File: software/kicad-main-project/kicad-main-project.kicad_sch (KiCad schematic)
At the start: 24 parts, among them J1 MOTOR_A, J2 MOTOR_B, SW1 SW_Push, SW2 SW_Push, SW3 SW_Push, SW4 SW_Push, U1 ESP32-DevKitC, U2 AMS117-5V, U3 TB6612FNG, U4 GP2Y0A02YK0F_1, U5 GP2Y0A02YK0F_2, U6 LCD-I2C, U7 CH340E

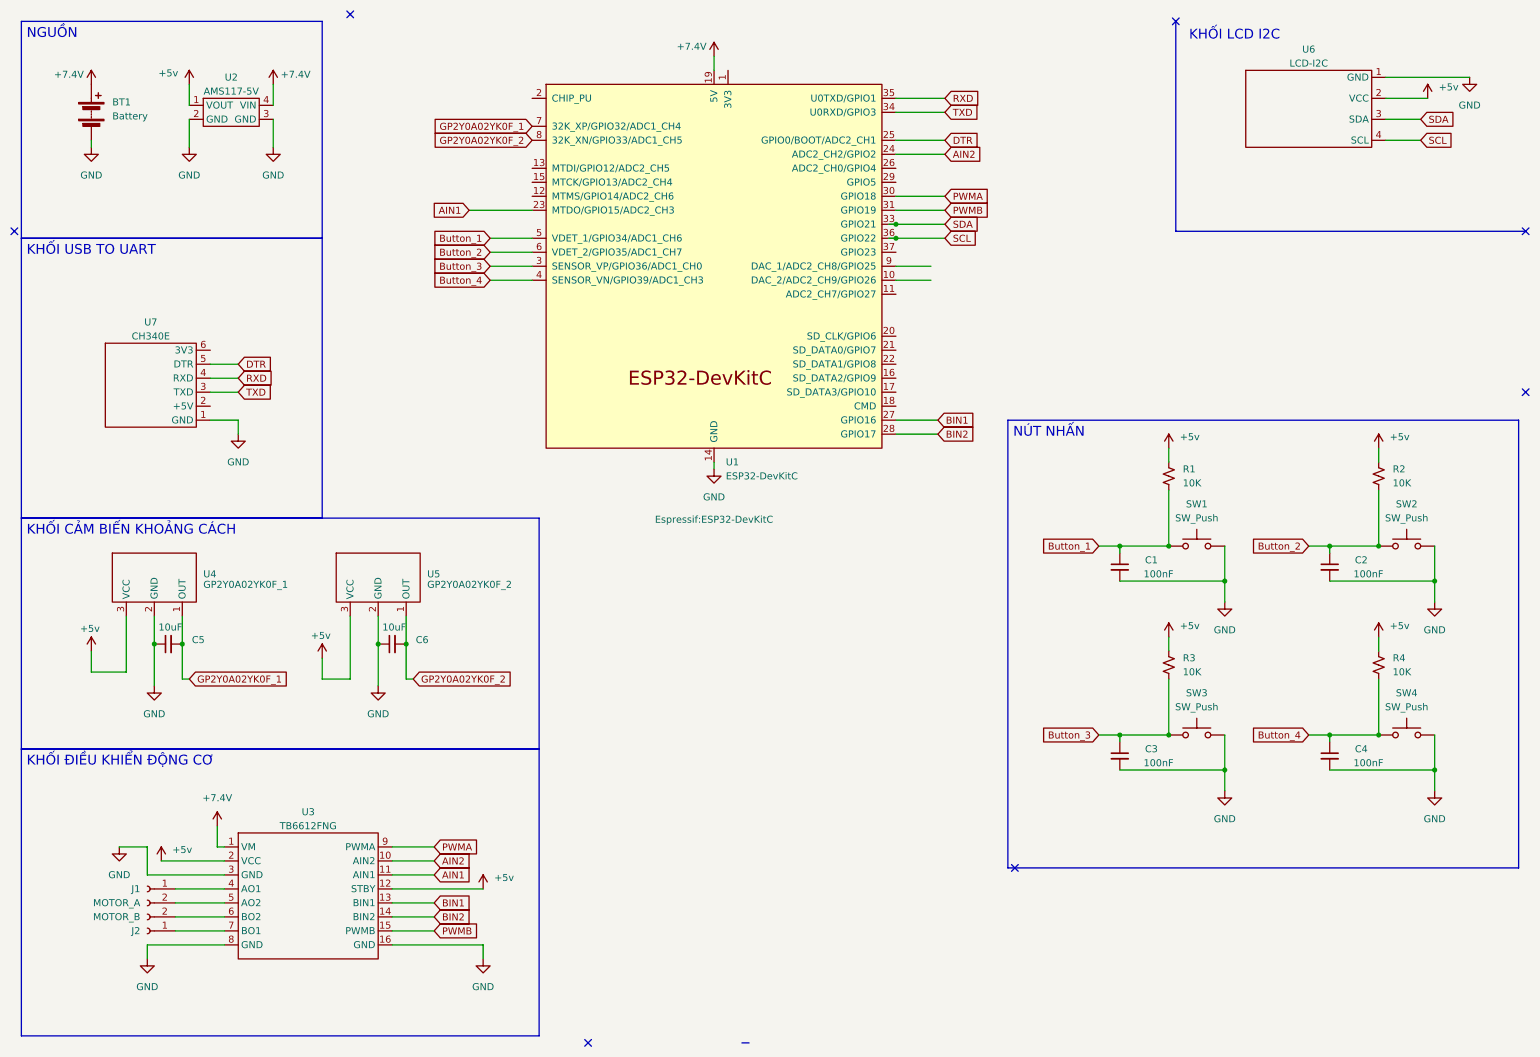
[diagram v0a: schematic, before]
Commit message: update gerber + bom + image_
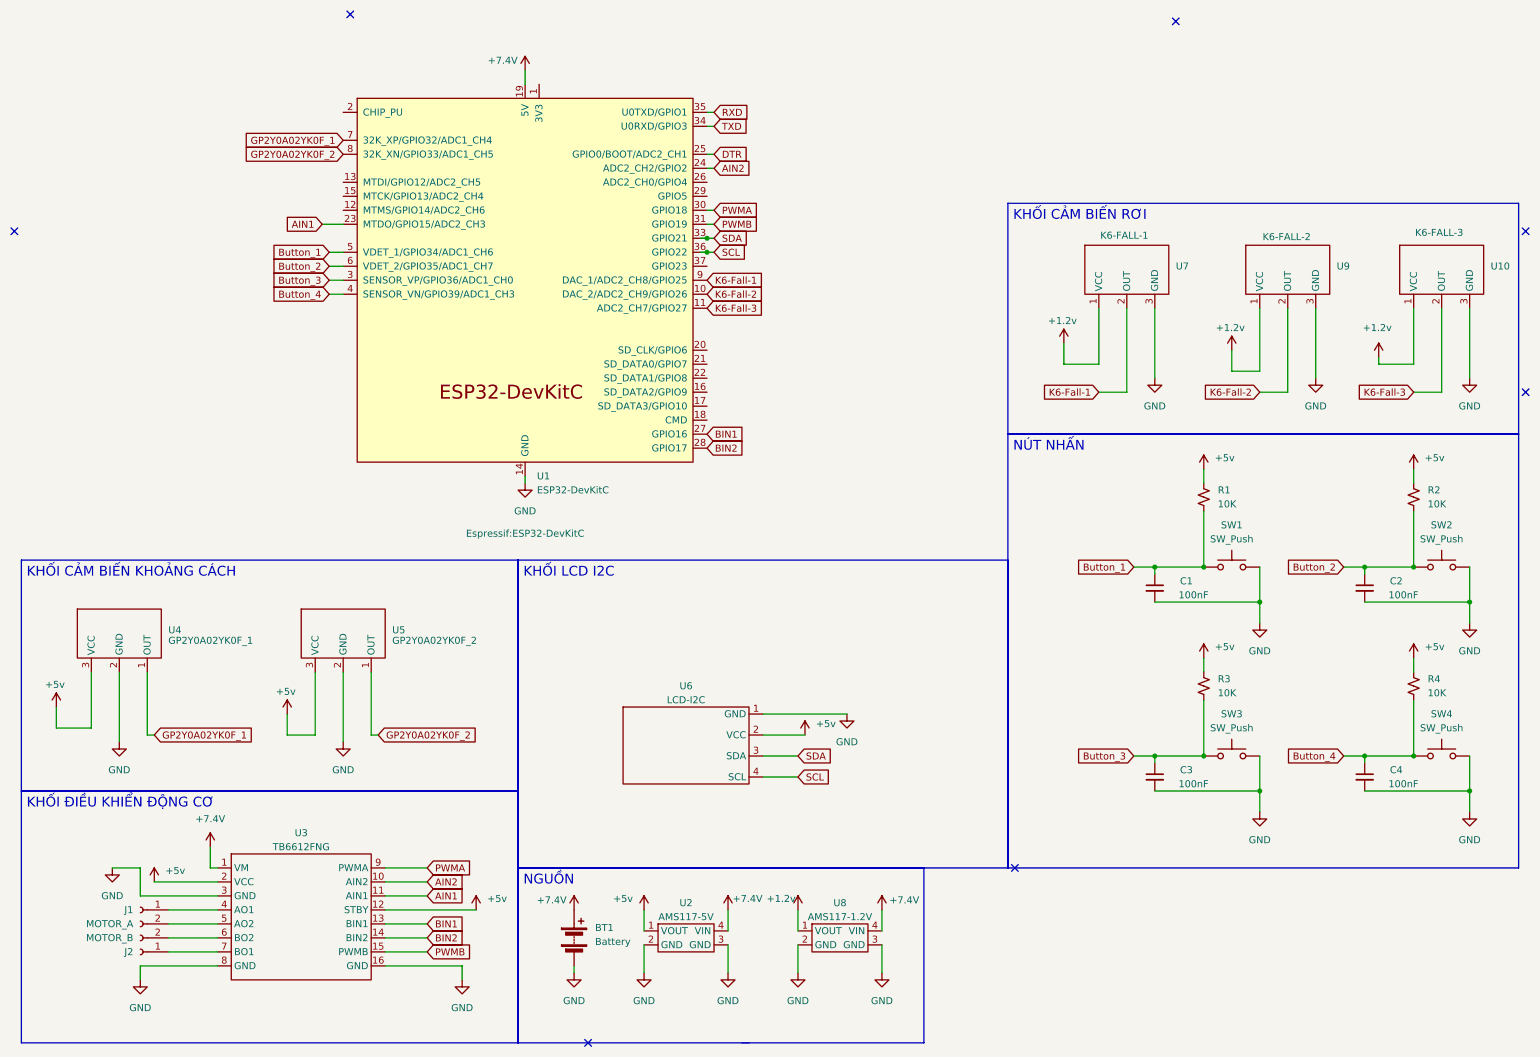
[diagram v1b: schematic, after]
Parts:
- removed C5, C6: 10uF, Capacitor_THT:C_Disc_D3.0mm_W1.6mm_P2.50mm, symbol Device:C_Small
- removed U7: CH340E, myCH340e:Untitled, symbol myCH340E:CH340E
- added U10: K6-FALL-3, Connector_JST:JST_XH_S3B-XH-A-1_1x03_P2.50mm_Horizontal, symbol myK6-Fall:K6-Fall
- added U7: K6-FALL-1, Connector_JST:JST_XH_S3B-XH-A-1_1x03_P2.50mm_Horizontal, symbol myK6-Fall:K6-Fall
- added U8: AMS117-1.2V, myAMS117-5V:Untitled, symbol myAMS117-1V2-Module:myAMS117-1V2
- added U9: K6-FALL-2, Connector_JST:JST_XH_S3B-XH-A-1_1x03_P2.50mm_Horizontal, symbol myK6-Fall:K6-Fall
- R1, R2, R3, R4: footprint Resistor_THT:R_Axial_DIN0617_L17.0mm_D6.0mm_P25.40mm_Horizontal -> Resistor_THT:R_Axial_DIN0204_L3.6mm_D1.6mm_P2.54mm_Vertical
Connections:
- net +7.4V: now also U8.4 (VIN)
- net GND: now also U10.3 (GND), U7.3 (GND), U8.2 (GND), U8.3 (GND), U9.3 (GND)
- net K6-Fall-2: now reaches U1.10 (DAC_2/ADC2_CH9/GPIO26)
- net K6-Fall-2: now also U9.2 (OUT)
- net K6-Fall-3: now reaches U1.11 (ADC2_CH7/GPIO27)
- net K6-Fall-3: now also U10.2 (OUT)
- net K6-Fall-1: now reaches U1.9 (DAC_1/ADC2_CH8/GPIO25)
- net K6-Fall-1: now also U7.2 (OUT)
- new net +1.2v: U10.1 (VCC), U7.1 (VCC), U8.1 (VOUT), U9.1 (VCC)
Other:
- note removed: "KHỐI LCD I2C"
- moved on the sheet: BT1, C1, C2, C3, C4, J1, J2, R1, R2, R3, R4, SW1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
